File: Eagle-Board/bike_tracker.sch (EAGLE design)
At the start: 69 parts, among them J1 TRANSFLASH-LOCK, Q1 IRLML5203, Q2 IRLML5203, Q3 IRLML5203, Q4 IRLML5203

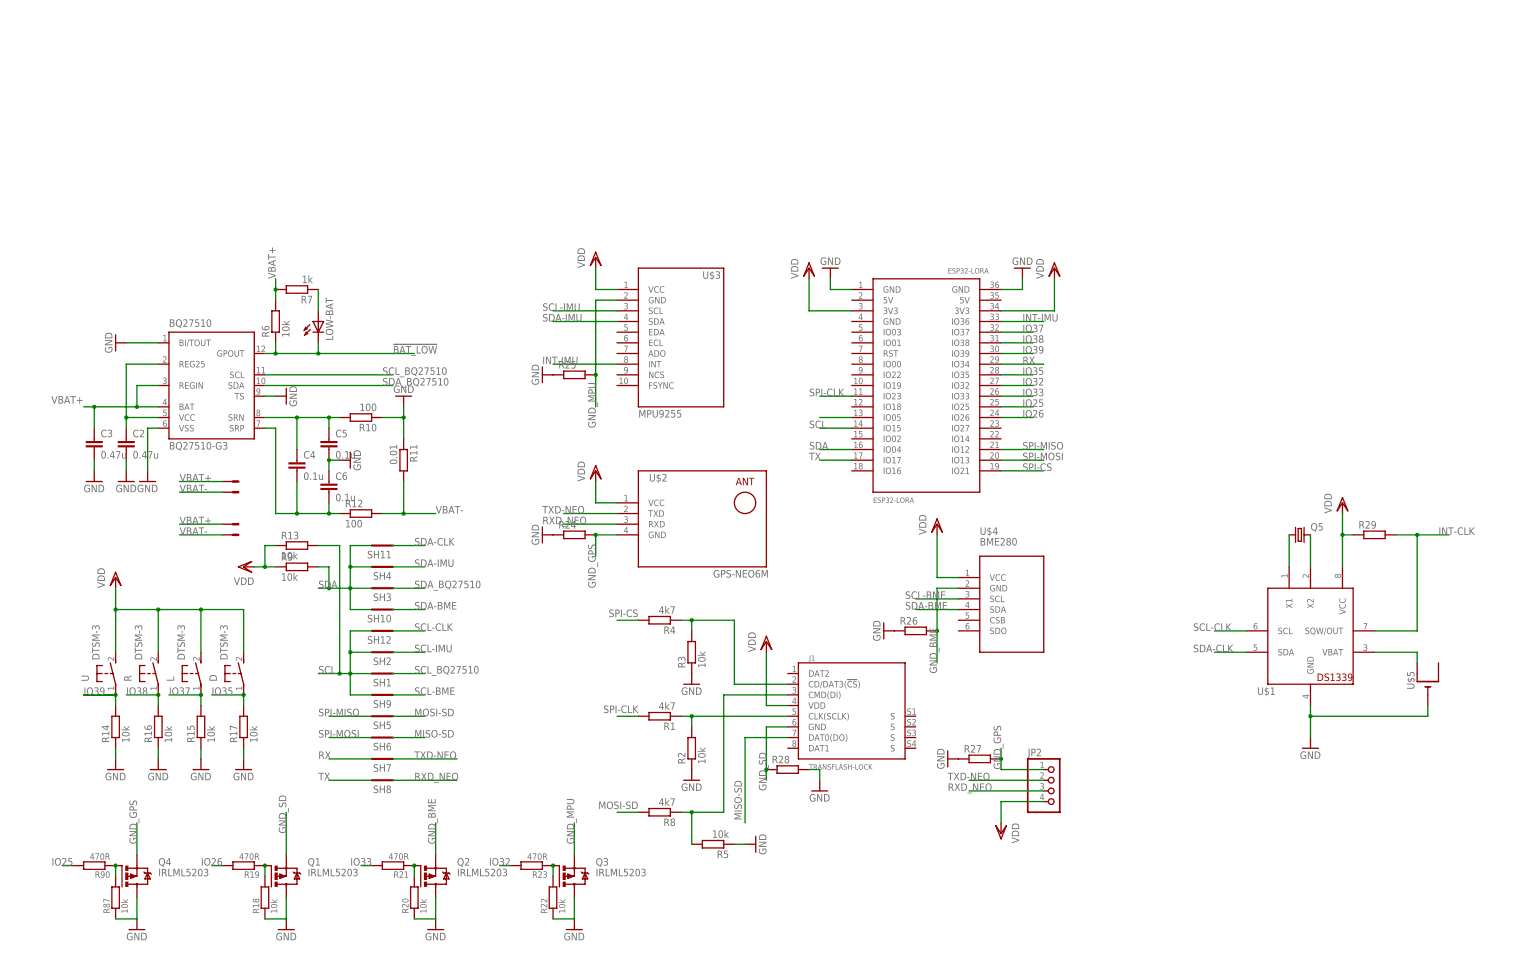
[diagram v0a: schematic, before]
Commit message: revision v1.2
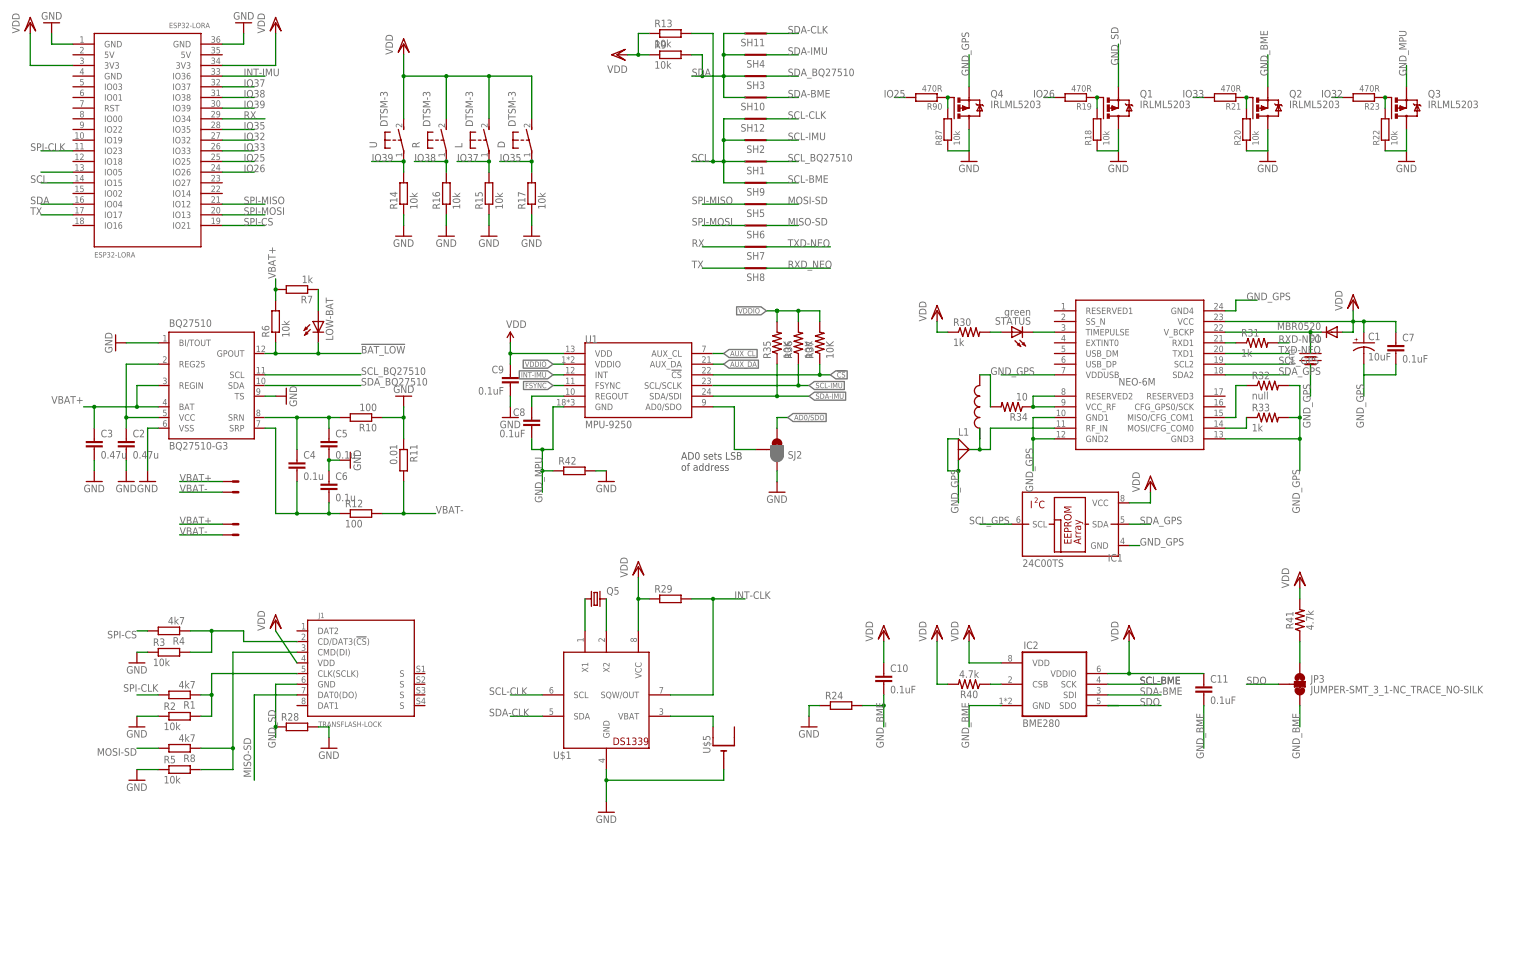
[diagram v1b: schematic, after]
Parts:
- removed JP2: (no value), pinhead:PINHD-1X4
- removed R25, R26, R27: (no value), resistor:R-EU_R0201
- removed U$2: GPS-NEO6M, diy-modules:GPS-NEO6M
- removed U$3: MPU9255, diy-modules:MPU9255
- removed U$4: BME280, diy-modules:BME280
- added BAT1: XH414, microduino:BATTERY-TS414H
- added C1: 10uF, microduino:CAP_POL3528
- added C10, C11: 0.1uF, SparkFun-Capacitors:0.1UF-0603-25V-(+80/-20%)
- added C7: 0.1uF, microduino:CAP0603-CAP
- added C8, C9: 0.1uF, SparkFun-Capacitors:0.1UF-25V(+80/-20%)(0603)
- added D1: MBR0520, microduino:DIODE-SOD123
- added IC1: 24C00TS, microchip:24C00TS
- added IC2: BME280, bosch-bme280:BME280
- added IPEX: ANT-UMCC, microduino:ANT-UMCC
- added JP3: JUMPER-SMT_3_1-NC_TRACE_NO-SILK, SparkFun-Jumpers:JUMPER-SMT_3_1-NC_TRACE_NO-SILK
- added L1: (no value), microduino:INDUCTOR0603
- added R30, R31, R33: 1k, microduino:RESISTOR0603-RES
- added R32: null, microduino:RESISTOR0603-RES
- added R34: 10, microduino:RESISTOR0603-RES
- added R35, R36, R37: 10K, SparkFun-Resistors:10KOHM-1/10W-1%(0603)0603
- added R40, R41: 4.7k, SparkFun-Resistors:4.7KOHM-0603-1/10W-1%
- added R42: (no value), resistor:R-EU_R0201
- added SJ2: JUMPER_PAD-3-1&2_NC_BY_PASTE, SparkFun-Passives:JUMPER_PAD-3-1&2_NC_BY_PASTE
- added STATUS: green, microduino:LED0805
- added U$6: BLOX-NEO-6M, microduino:BLOX-NEO-6M
- added U1: MPU-9250, Testing:MPU-9250
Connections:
- new net !CS: R37.1, U1.!CS
- new net AD0/SDO: SJ2.3
- new net ADSD_STUB: SJ2.2, U1.AD0/SDO
- new net AUX_CL: U1.AUX_CL
- new net AUX_DA: U1.AUX_DA
- new net FSYNC: U1.FSYNC
- new net N$16: R30.2, STATUS.A
- new net N$17: STATUS.C, U$6.TIMEPULSE
- new net N$18: IPEX.ANT, L1.1, U$6.RF_IN
- new net N$19: R31.1, U$6.RXD1
- new net N$20: R32.1, U$6.MISO/CFG_COM1
- new net N$21: R33.1, U$6.MOSI/CFG_COM0
- new net N$22: BAT1.+, D1.C, U$6.V_BCKP
- new net N$23: L1.2, R34.2
- new net N$24: R34.1, U$6.RESERVED2, U$6.VCC_RF
- new net N$25: IC2.CSB, R40.1
- new net N$26: JP3.1, R41.1
- new net REGOUT: C8.1, U1.REGOUT
- new net RXD-NEO: R31.2
- new net SCL_GPS: IC1.SCL, U$6.SCL2
- new net SDA_GPS: IC1.SDA, U$6.SDA2
- new net SDO: IC2.SDO, JP3.2
- new net VDDIO: R35.2, R36.2, R37.2, U1.VDDIO
- net GND: now also C9.2, R42.2, SJ2.1; no longer R25.1, R26.1, R27.1
- net GND_BME: now also C10.2, C11.2, IC2.GND, JP3.3, R24.2; no longer R26.2, U$4.GND
- net GND_GPS: now also BAT1.-, C1.-, C7.2, IC1.GND, IPEX.GND1, IPEX.GND2, R32.2, R33.2, U$6.GND1, U$6.GND2, U$6.GND3, U$6.GND4, U$6.VDDUSB; no longer JP2.1, R24.2, R27.2, U$2.GND
- net GND_MPU: now also C8.2, R42.1, U1.GND; no longer R25.2, U$3.GND
- net INT-IMU: now also U1.INT; no longer U$3.INT
- net RXD_NEO: no longer JP2.3, U$2.RXD
- net SCL-BME: now also IC2.SCK; no longer U$4.SCL
- net SCL-IMU: now also R36.1, U1.SCL/SCLK; no longer U$3.SCL
- net SDA-BME: now also IC2.SDI; no longer U$4.SDA
- net SDA-IMU: now also R35.1, U1.SDA/SDI; no longer U$3.SDA
- net TXD-NEO: now also U$6.TXD1; no longer JP2.2, U$2.TXD
- net VDD: now also C1.+, C10.1, C11.1, C7.1, C9.1, D1.A, IC1.VCC, IC2.VDD, IC2.VDDIO, R30.1, R40.2, R41.2, U$6.VCC, U1.VDD; no longer JP2.4, U$2.VCC, U$3.VCC, U$4.VCC
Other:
- note added: "AD0 sets LSB of address"
- moved on the sheet: D, ESP32-LORA, J1, L, Q1, Q2, Q3, Q4, Q5, R, R1, R13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
